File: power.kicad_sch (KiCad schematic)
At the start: 251 parts, among them J3 Conn_01x01, J4 Conn_01x01, U1 CSD95472Q5MC, U16 CSD95472Q5MC, U18 CSD95472Q5MC, U19 CSD95472Q5MC, U3 TPS53667, U36 MCP1824T-1202E, U4 CSD95472Q5MC, U5 CSD95472Q5MC, U6 AP3211, U7 MCP1824T-0802E

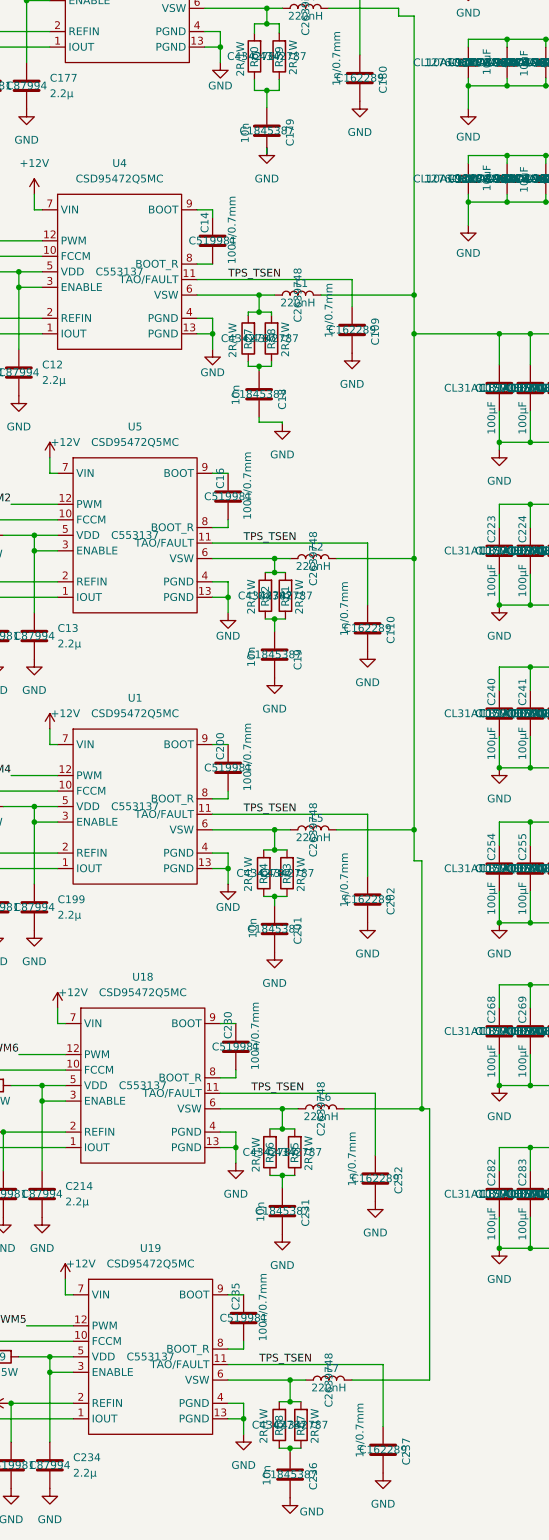
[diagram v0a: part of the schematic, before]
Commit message: Rev3.4
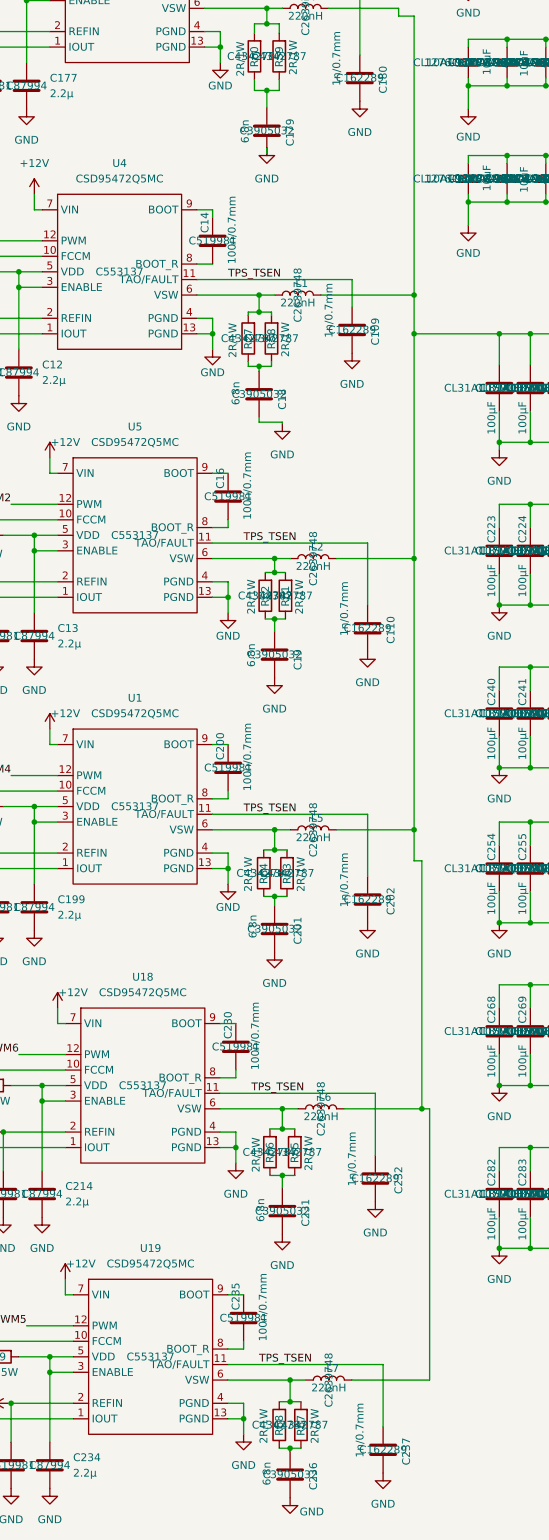
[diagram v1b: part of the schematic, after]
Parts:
- C179, C18, C19, C201, C231, C236: value 10n -> 6.8n; LCSC Part # C1845387 -> C3905032; Manufacturer CGA4C2C0G1H103J060AA -> GRM2165C2A682JA01D; OrderNr 445-6947-1-ND -> 490-GRM2165C2A682JA01DCT-ND
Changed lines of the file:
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@@
 			)
 		)
-		(property "Value" "10n"
+		(property "Value" "6.8n"
 			(at 231.394 58.928 90)
 			(effects
@@
 			)
 		)
-		(property "Description" "CAP CER 10000PF 50V C0G 0805"
+		(property "Description" "CAP CER 6800PF 100V C0G/NP0 0805"
 			(at 234.95 56.896 0)
 			(effects
@@
 			)
 		)
-		(property "Manufacturer" "CGA4C2C0G1H103J060AA"
+		(property "Manufacturer" "GRM2165C2A682JA01D"
 			(at 234.95 56.896 0)
 			(effects
@@
 			)
 		)
-		(property "OrderNr" "445-6947-1-ND"
+		(property "OrderNr" "490-GRM2165C2A682JA01DCT-ND"
 			(at 234.95 56.896 0)
 			(effects
@@
 			)
 		)
-		(property "LCSC Part #" "C1845387"
+		(property "LCSC Part #" "C3905032"
 			(at 234.95 56.896 0)
 			(effects
@@
 			)
 		)
-		(property "Value" "10n"
+		(property "Value" "6.8n"
 			(at 234.95 278.892 90)
 			(effects
@@
 			)
 		)
-		(property "Description" "CAP CER 10000PF 50V C0G 0805"
+		(property "Description" "CAP CER 6800PF 100V C0G/NP0 0805"
 			(at 238.76 277.114 0)
 			(effects
@@
 			)
 		)
-		(property "Manufacturer" "CGA4C2C0G1H103J060AA"
+		(property "Manufacturer" "GRM2165C2A682JA01D"
 			(at 238.76 277.114 0)
 			(effects
@@
 			)
 		)
-		(property "OrderNr" "445-6947-1-ND"
+		(property "OrderNr" "490-GRM2165C2A682JA01DCT-ND"
 			(at 238.76 277.114 0)
 			(effects
@@
 			)
 		)
-		(property "LCSC Part #" "C1845387"
+		(property "LCSC Part #" "C3905032"
 			(at 238.76 277.114 0)
 			(effects
@@
 			)
 		)
-		(property "Value" "10n"
+		(property "Value" "6.8n"
 			(at 229.87 101.854 90)
 			(effects
@@
 			)
 		)
-		(property "Description" "CAP CER 10000PF 50V C0G 0805"
+		(property "Description" "CAP CER 6800PF 100V C0G/NP0 0805"
 			(at 233.68 100.076 0)
 			(effects
@@
 			)
 		)
-		(property "Manufacturer" "CGA4C2C0G1H103J060AA"
+		(property "Manufacturer" "GRM2165C2A682JA01D"
 			(at 233.68 100.076 0)
 			(effects
@@
 			)
 		)
-		(property "OrderNr" "445-6947-1-ND"
+		(property "OrderNr" "490-GRM2165C2A682JA01DCT-ND"
 			(at 233.68 100.076 0)
 			(effects
@@
 			)
 		)
-		(property "LCSC Part #" "C1845387"
+		(property "LCSC Part #" "C3905032"
 			(at 233.68 100.076 0)
 			(effects
@@
 			)
 		)
-		(property "Value" "10n"
+		(property "Value" "6.8n"
 			(at 232.41 144.78 90)
 			(effects
@@
 			)
 		)
-		(property "Description" "CAP CER 10000PF 50V C0G 0805"
+		(property "Description" "CAP CER 6800PF 100V C0G/NP0 0805"
 			(at 236.22 142.748 0)
 			(effects
@@
 			)
 		)
-		(property "Manufacturer" "CGA4C2C0G1H103J060AA"
+		(property "Manufacturer" "GRM2165C2A682JA01D"
 			(at 236.22 142.748 0)
 			(effects
@@
 			)
 		)
-		(property "OrderNr" "445-6947-1-ND"
+		(property "OrderNr" "490-GRM2165C2A682JA01DCT-ND"
 			(at 236.22 142.748 0)
 			(effects
@@
 			)
 		)
-		(property "LCSC Part #" "C1845387"
+		(property "LCSC Part #" "C3905032"
 			(at 236.22 142.748 0)
 			(effects
@@
 			)
 		)
-		(property "Value" "10n"
+		(property "Value" "6.8n"
 			(at 233.934 235.712 90)
 			(effects
@@
 			)
 		)
-		(property "Description" "CAP CER 10000PF 50V C0G 0805"
+		(property "Description" "CAP CER 6800PF 100V C0G/NP0 0805"
 			(at 237.49 233.934 0)
 			(effects
@@
 			)
 		)
-		(property "Manufacturer" "CGA4C2C0G1H103J060AA"
+		(property "Manufacturer" "GRM2165C2A682JA01D"
 			(at 237.49 233.934 0)
 			(effects
@@
 			)
 		)
-		(property "OrderNr" "445-6947-1-ND"
+		(property "OrderNr" "490-GRM2165C2A682JA01DCT-ND"
 			(at 237.49 233.934 0)
 			(effects
@@
 			)
 		)
-		(property "LCSC Part #" "C1845387"
+		(property "LCSC Part #" "C3905032"
 			(at 237.49 233.934 0)
 			(effects
@@
 			)
 		)
-		(property "Value" "10n"
+		(property "Value" "6.8n"
 			(at 232.664 189.23 90)
 			(effects
@@
 			)
 		)
-		(property "Description" "CAP CER 10000PF 50V C0G 0805"
+		(property "Description" "CAP CER 6800PF 100V C0G/NP0 0805"
 			(at 236.22 187.706 0)
 			(effects
@@
 			)
 		)
-		(property "Manufacturer" "CGA4C2C0G1H103J060AA"
+		(property "Manufacturer" "GRM2165C2A682JA01D"
 			(at 236.22 187.706 0)
 			(effects
@@
 			)
 		)
-		(property "OrderNr" "445-6947-1-ND"
+		(property "OrderNr" "490-GRM2165C2A682JA01DCT-ND"
 			(at 236.22 187.706 0)
 			(effects
@@
 			)
 		)
-		(property "LCSC Part #" "C1845387"
+		(property "LCSC Part #" "C3905032"
 			(at 236.22 187.706 0)
 			(effects
